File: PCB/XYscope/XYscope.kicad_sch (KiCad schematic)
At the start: 11 parts, among them J1 Power, J2 Digital/PWM, J3 Analog, J4 Digital/PWM, J5 Conn_01x06_Socket, J6 Conn_01x06_Socket, J7 Conn_01x06_Socket, J8 CONBNC002, J9 CONBNC002

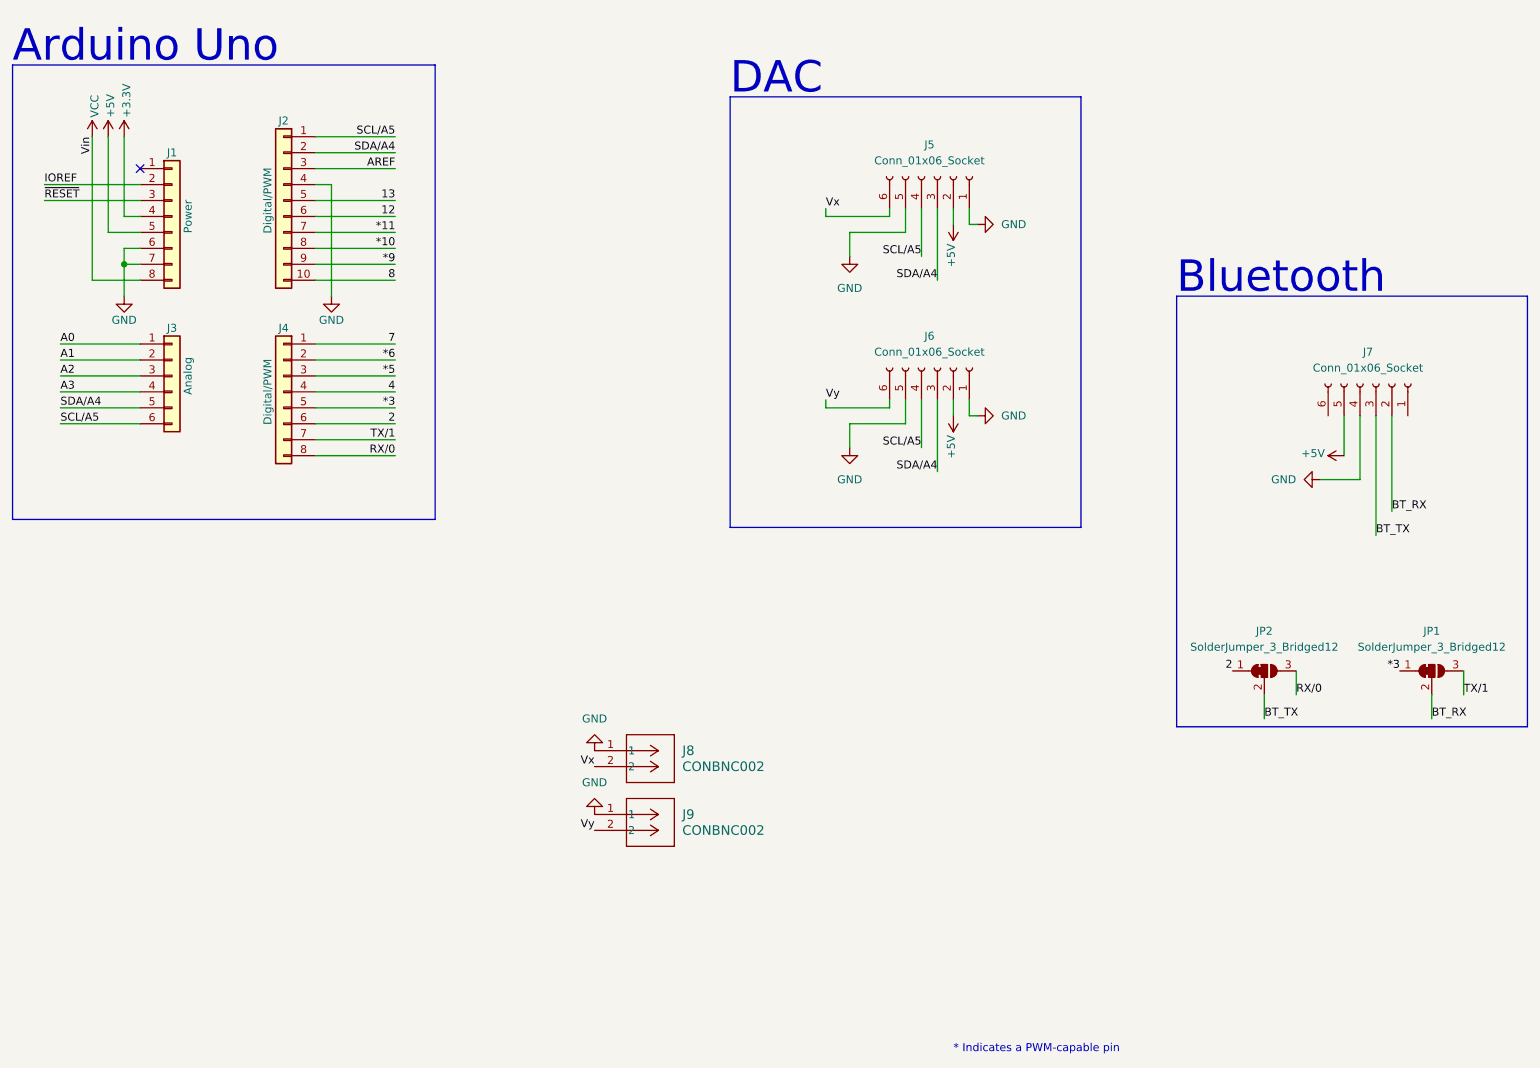
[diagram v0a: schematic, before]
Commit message: Added pictures
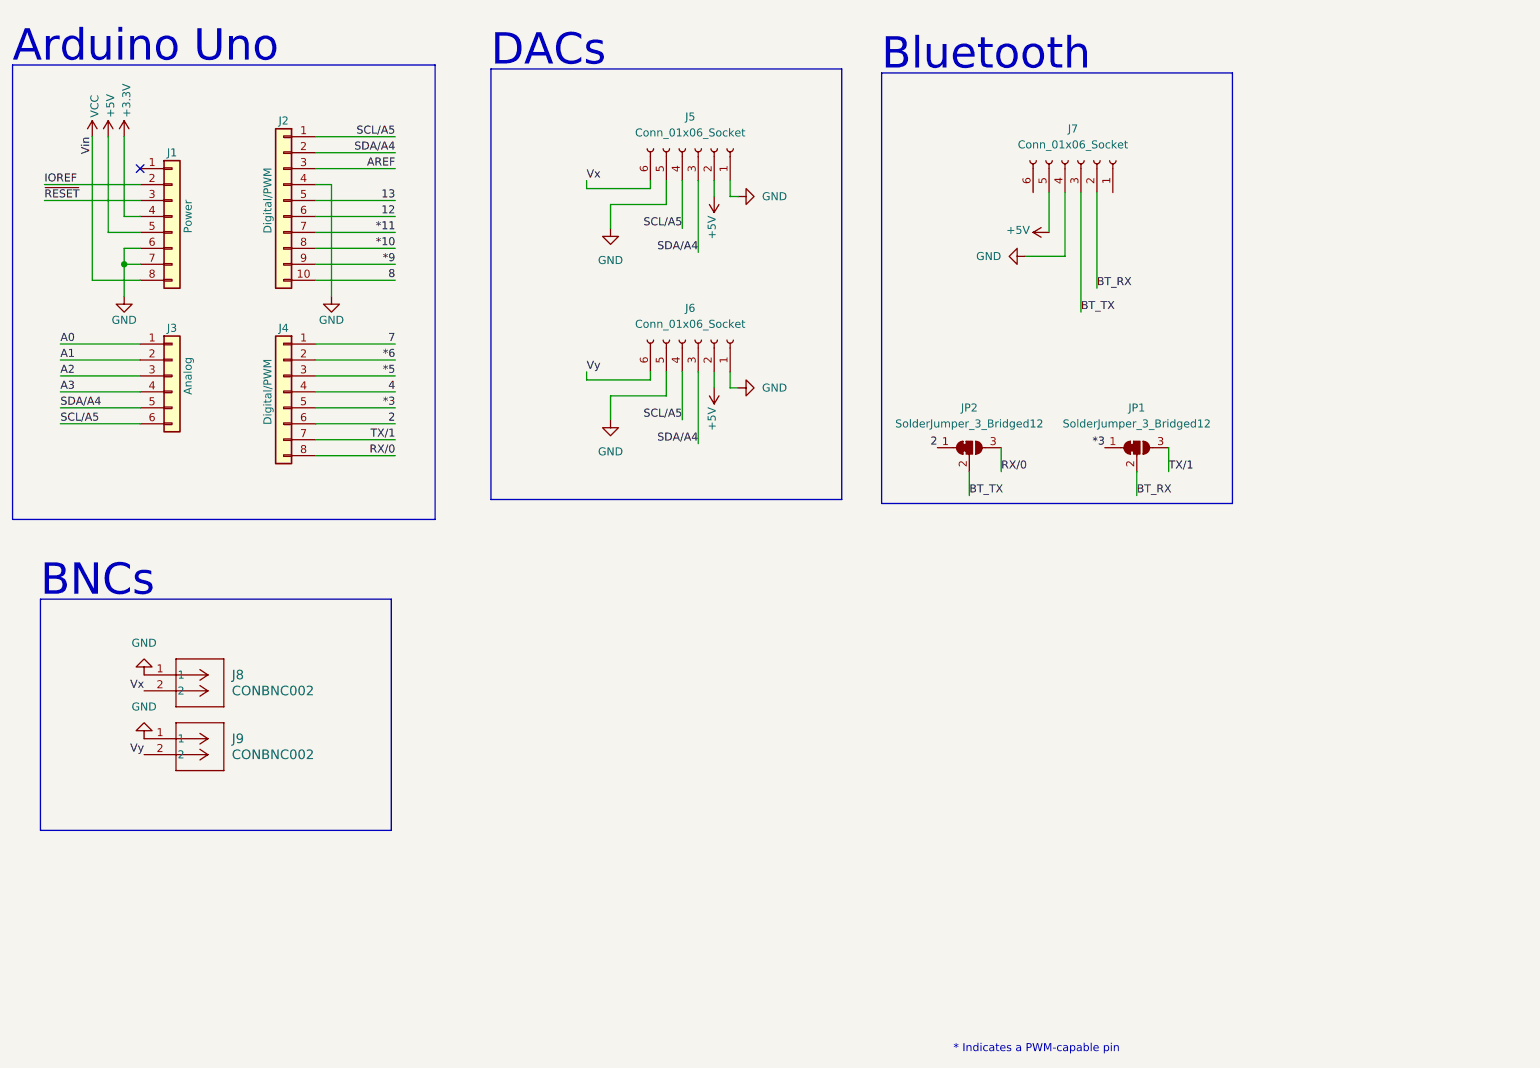
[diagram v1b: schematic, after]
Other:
- note added: "BNCs"
- note added: "DACs"
- note removed: "DAC"
- moved on the sheet: J5, J6, J7, J8, J9, JP1, JP2
